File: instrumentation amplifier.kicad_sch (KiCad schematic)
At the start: 13 parts, among them J1 Conn_02x02_Odd_Even, J2 Conn_02x01, J3 Conn_02x01, U1 TL074

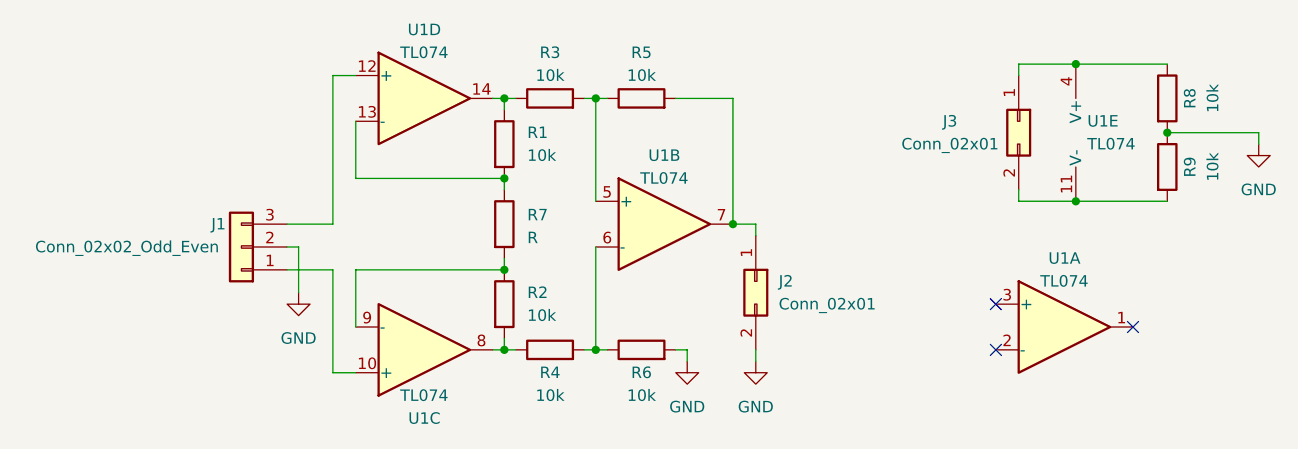
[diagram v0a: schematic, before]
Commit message: release v1
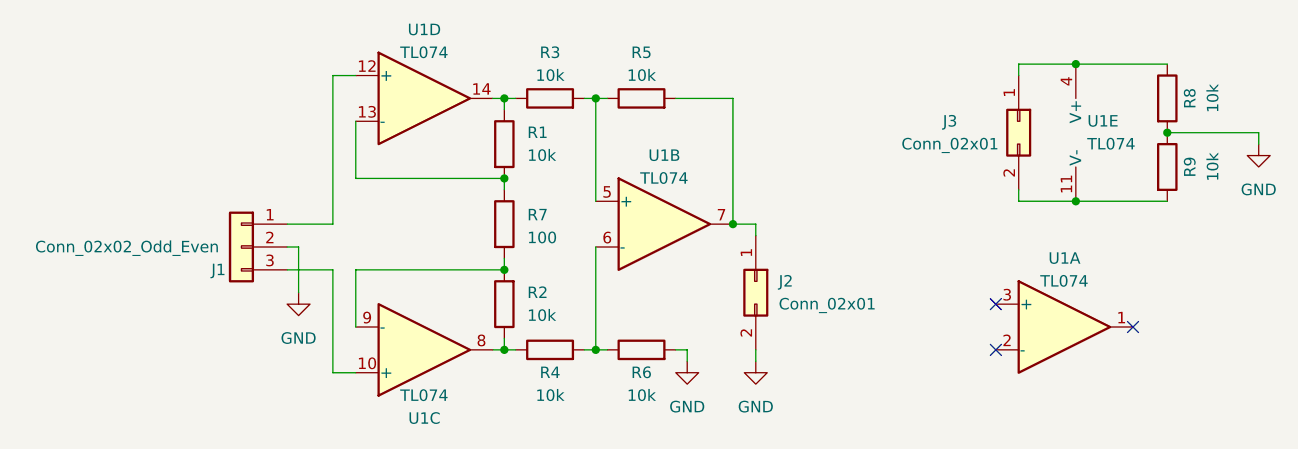
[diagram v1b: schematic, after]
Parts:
- R7: value R -> 100
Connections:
- net at U1.10 (+): now also J1.3 (Pin_3); no longer J1.1 (Pin_1)
- net at R4.1, U1.8: now also R2.1; no longer R2.2
- net at R7.2, U1.9 (-): now also R2.2; no longer R2.1
- net at U1.12 (+): now also J1.1 (Pin_1); no longer J1.3 (Pin_3)
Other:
- moved on the sheet: J1, R2
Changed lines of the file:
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@@
 	(title_block
 		(title "Instrumentation amplifier board")
+		(date "2025-08-23")
 		(rev "1")
 	)
@@
 	(symbol
 		(lib_id "Device:R")
-		(at 128.27 101.6 0)
+		(at 128.27 101.6 180)
 		(unit 1)
 		(exclude_from_sim no)
@@
 		(on_board yes)
 		(dnp no)
-		(fields_autoplaced yes)
 		(property "Reference" "R2"
 			(at 130.81 100.3299 0)
@@
 					(size 1.27 1.27)
 				)
-				(justify left)
+				(justify right)
 			)
 		)
@@
 					(size 1.27 1.27)
 				)
-				(justify left)
+				(justify right)
 			)
 		)
 		(property "Footprint" "Resistor_SMD:R_1206_3216Metric_Pad1.30x1.75mm_HandSolder"
-			(at 126.492 101.6 90)
+			(at 130.048 101.6 90)
 			(effects
 				(font
@@
 	(symbol
 		(lib_id "Connector_Generic:Conn_01x03")
-		(at 99.06 95.25 180)
+		(at 99.06 95.25 0)
+		(mirror y)
 		(unit 1)
 		(exclude_from_sim no)
@@
 		(dnp no)
 		(property "Reference" "J1"
-			(at 96.52 92.71 0)
+			(at 96.52 97.79 0)
 			(effects
 				(font
@@
 			)
 		)
-		(property "Value" "R"
+		(property "Value" "100"
 			(at 130.81 94.234 0)
 			(effects
